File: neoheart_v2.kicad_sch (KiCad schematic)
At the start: 44 parts, among them J1 Conn_01x03, Q1 A1SHB, Q2 BSS138, U2 TPS61240TDRVRQ1

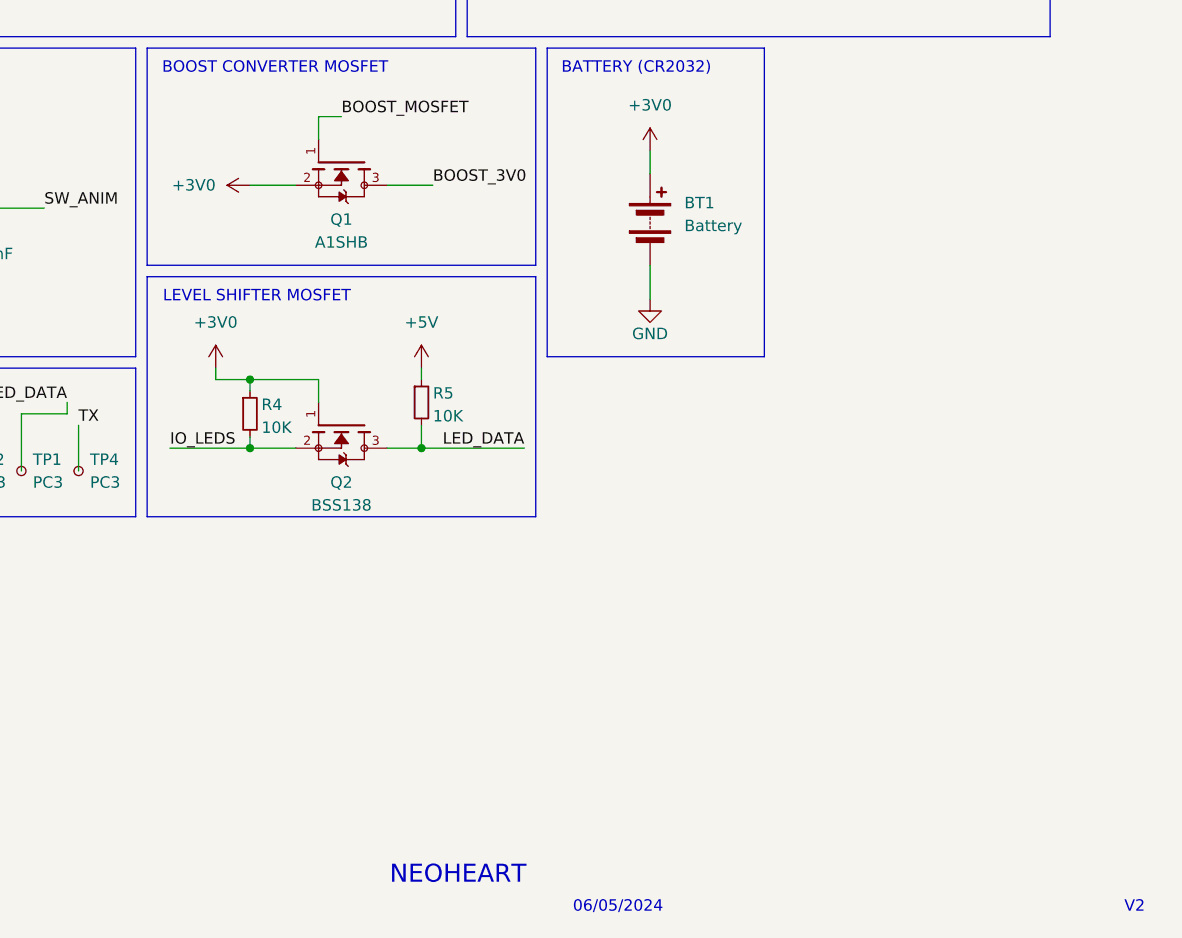
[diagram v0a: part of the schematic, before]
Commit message: revision 2.1, pcbway production files
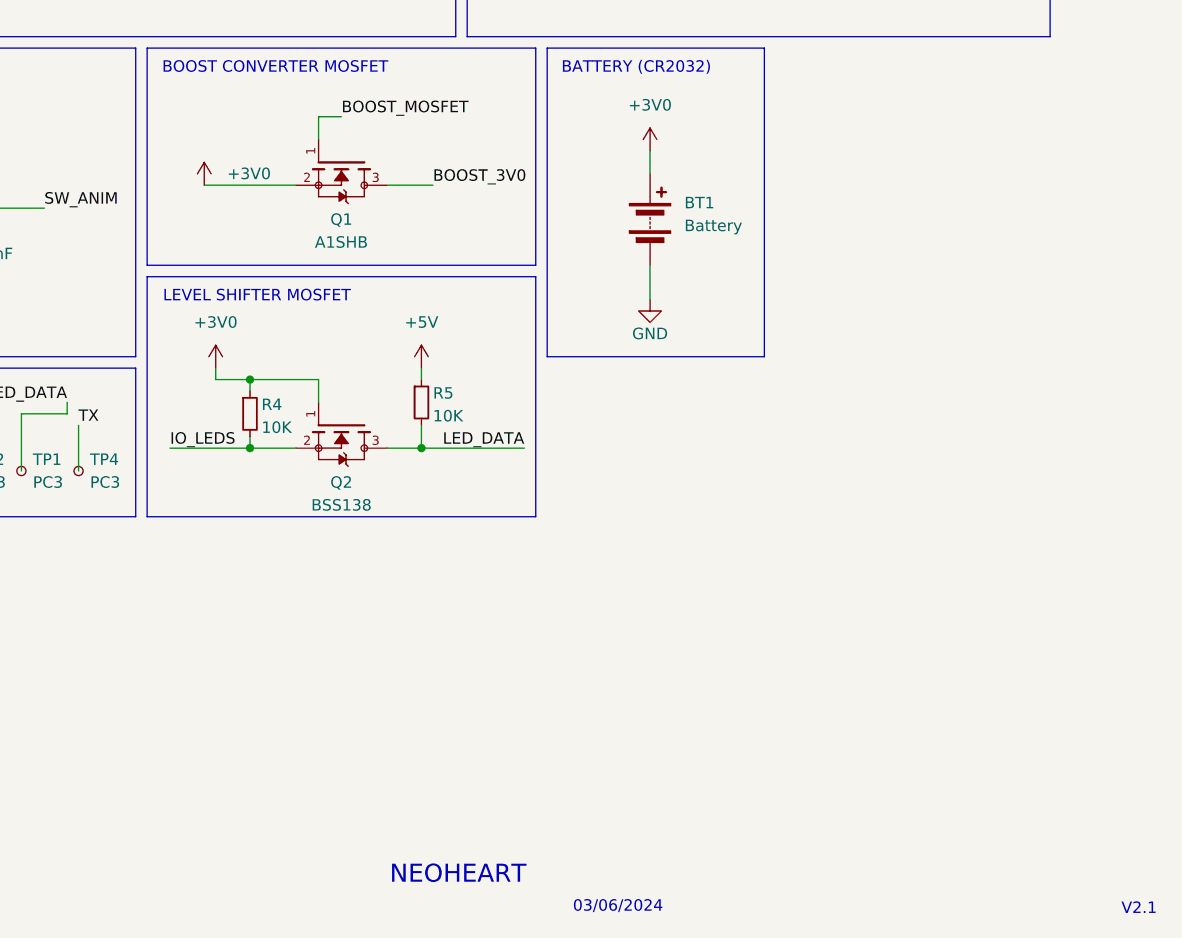
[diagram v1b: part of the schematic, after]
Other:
- note added: "03/06/2024"
- note added: "V2.1"
- note removed: "06/05/2024"
- note removed: "V2"
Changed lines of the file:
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@@
 	(wire
 		(pts
-			(xy 171.45 113.03) (xy 176.53 113.03)
+			(xy 166.37 113.03) (xy 176.53 113.03)
 		)
 		(stroke
@@
 		)
 	)
-	(text "06/05/2024"
+	(text "03/06/2024"
 		(exclude_from_sim no)
 		(at 212.344 193.294 0)
@@
 		)
 	)
-	(text "V2"
+	(text "V2.1"
 		(exclude_from_sim no)
-		(at 269.748 193.294 0)
+		(at 270.256 193.548 0)
 		(effects
 			(font
@@
 	(symbol
 		(lib_id "power:+3V0")
-		(at 171.45 113.03 90)
+		(at 166.37 113.03 0)
 		(unit 1)
 		(exclude_from_sim no)
@@
 		(fields_autoplaced yes)
 		(property "Reference" "#PWR04"
-			(at 175.26 113.03 0)
+			(at 166.37 116.84 0)
 			(effects
 				(font
@@
 		)
 		(property "Value" "+3V0"
-			(at 167.64 113.0299 90)
+			(at 168.91 111.7599 0)
 			(effects
 				(font
@@
 		)
 		(property "Footprint" ""
-			(at 171.45 113.03 0)
+			(at 166.37 113.03 0)
 			(effects
 				(font
@@
 		)
 		(property "Datasheet" ""
-			(at 171.45 113.03 0)
+			(at 166.37 113.03 0)
 			(effects
 				(font
@@
 		)
 		(property "Description" ""
-			(at 171.45 113.03 0)
+			(at 166.37 113.03 0)
 			(effects
 				(font
